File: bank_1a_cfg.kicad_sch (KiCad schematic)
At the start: 48 parts, among them J3 T8_JTAG, Q1 SSM3K37MFV, SW1 Reconfig, U8 T20Q144xx, U9 AT25FF081A-SSHN-B

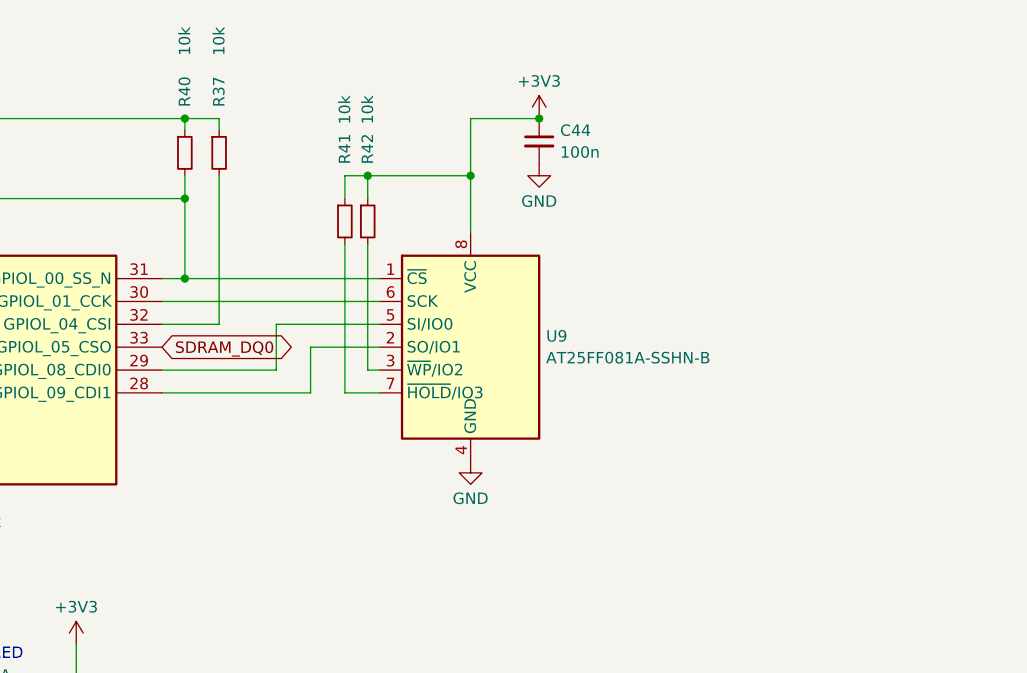
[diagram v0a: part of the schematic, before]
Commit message: reconnected fpgaGpio[0] from pin 36 -> 32 (REF_RES is *not* a GPIO!)
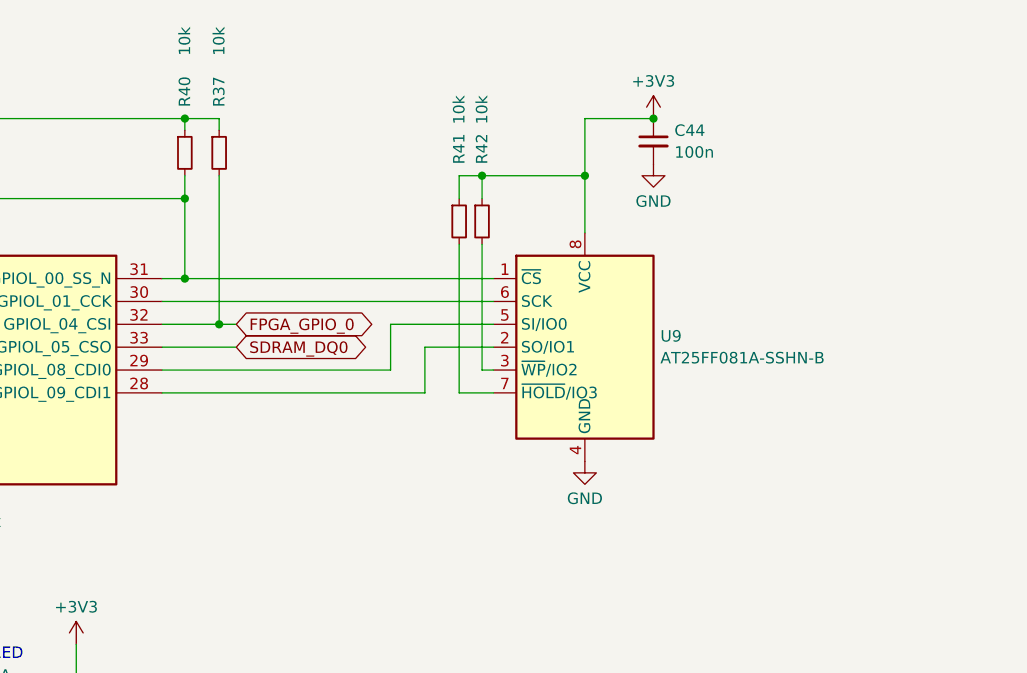
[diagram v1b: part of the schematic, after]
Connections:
- net FPGA_GPIO_0: now reaches R37.2, U8.32 (GPIOL_04_CSI)
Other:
- moved on the sheet: C44, R41, R42, U9
